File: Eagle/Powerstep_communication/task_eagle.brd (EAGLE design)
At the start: 82.5 x 123.6 mm, 104 parts, among them IC2 ATMEGA640-16AI, IC3 74ACT125D, IC7 FT232RL, IC8 MAX485, K1 G5LE, K2 G5LE, K3 G5LE, K6 G5LE, U1 TC1262-33VDB, U2 Tyco 5-6605758-1, U3 ENC28J60-SSOP, Y2 25MHz

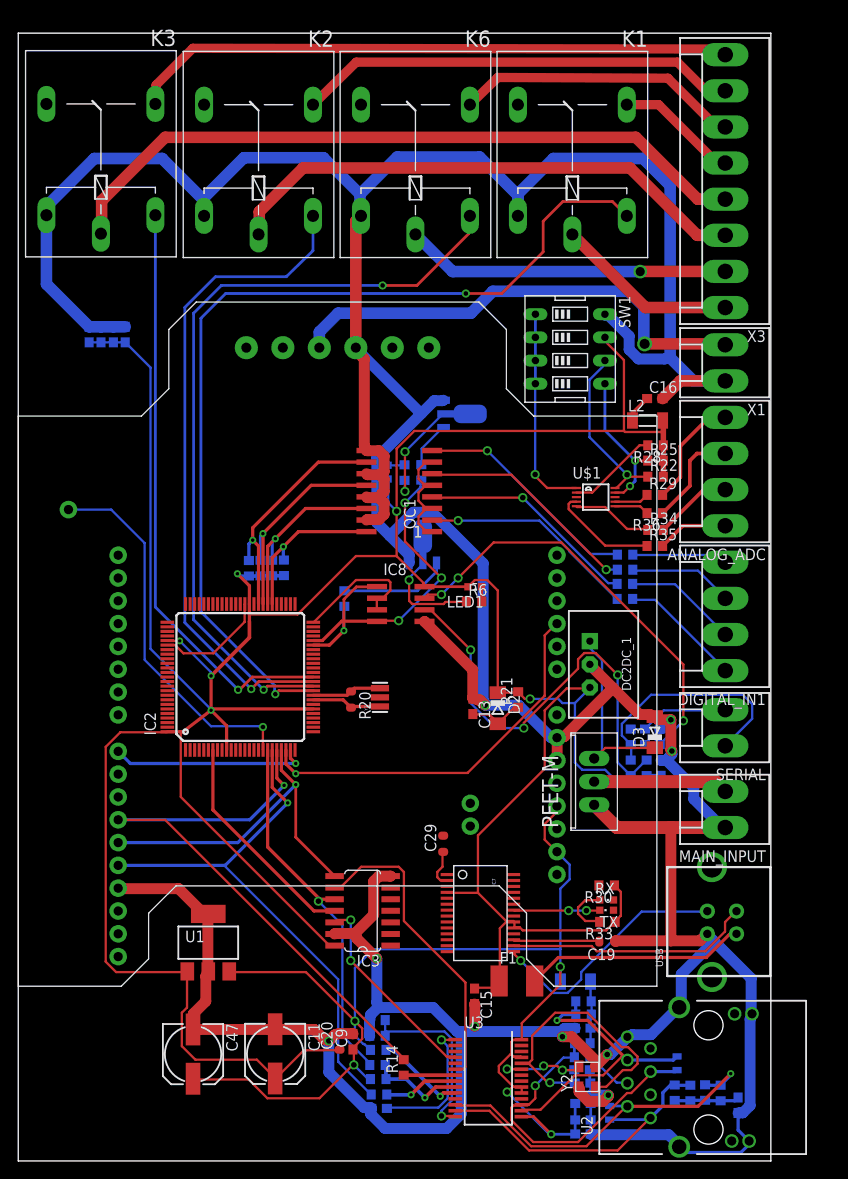
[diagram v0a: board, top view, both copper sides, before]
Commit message: eagle powerstepproto
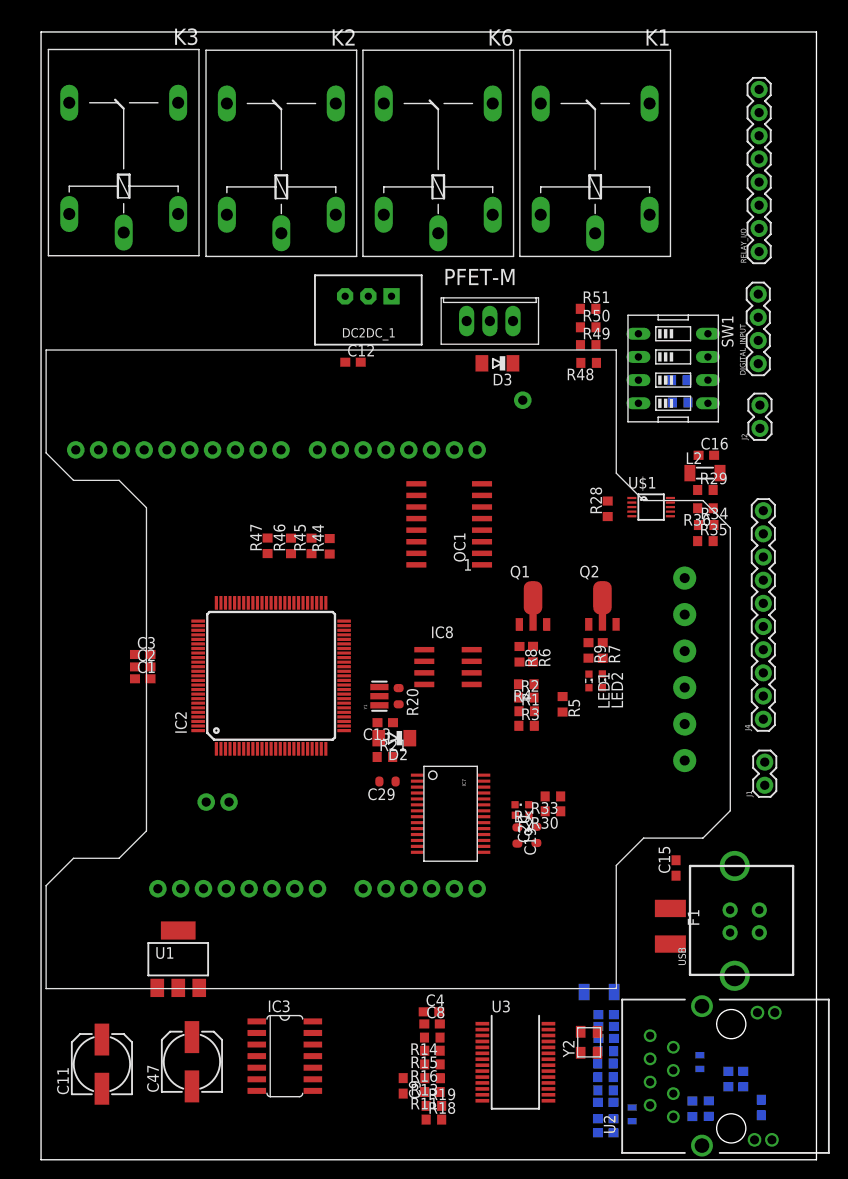
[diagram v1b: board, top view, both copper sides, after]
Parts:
- removed ANALOG_ADC, DIGITAL_IN1: (no value), con-molex:KK-156-4
- removed MAIN_INPUT, SERIAL, X1: (no value), con-molex:KK-156-2
- removed X3: (no value), con-molex:KK-156-8
- added DIGITAL_INPUT: (no value), SparkFun-Connectors:1X04
- added J1, J2: (no value), SparkFun-Connectors:1X02
- added J4: (no value), SparkFun-Connectors:1X10
- added RELAY_I/O: (no value), SparkFun-Connectors:1X08
- moved C4 81.5 mm to (42.8, 16.2), flipped to the top, turned to 0 degrees
- moved U$2 69.9 mm to (0.49, 88.8), turned to 270 degrees
- moved PFET-M 59.8 mm to (44.1, 94.5), turned to 0 degrees
- moved C12 55.9 mm to (34.2, 87.4), flipped to the top, turned to 0 degrees
- moved DC2DC_1 46.6 mm to (35.9, 93.2), turned to 180 degrees
- moved D3 44.0 mm to (50.0, 87.3), turned to 180 degrees
- moved C1 38.2 mm to (11.1, 52.7), flipped to the top, turned to 0 degrees
- moved C2 36.7 mm to (11.1, 54.0), flipped to the top, turned to 0 degrees
- moved C3 35.2 mm to (11.1, 55.4), flipped to the top, turned to 0 degrees
- moved LED2 32.8 mm to (61.5, 52.5), flipped to the top
- moved C20 31.3 mm to (54.3, 35.6)
- moved R7 29.2 mm to (61.6, 55.8), flipped to the top, turned to 270 degrees
- moved R51 27.3 mm to (60.0, 93.3), flipped to the top
- moved R50 26.9 mm to (60.0, 91.3), flipped to the top
- moved R9 26.8 mm to (60.0, 55.8), flipped to the top
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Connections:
- new net N$19: J4.1, U$2.A+
- new net N$33: J4.2, U$2.B+
- new net N$34: J4.5, U$2.B-
- new net N$35: J4.6, U$2.A-
- net 12V_IN: now also J2.2; no longer MAIN_INPUT.2
- net A: now also J1.1; no longer SERIAL.1
- net A0_ADC: now also J4.7; no longer ANALOG_ADC.1
- net A1_ADC: now also J4.8; no longer ANALOG_ADC.2
- net A2_ADC: now also J4.9; no longer ANALOG_ADC.3
- net A3_ADC: now also J4.10; no longer ANALOG_ADC.4
- net B: now also J1.2; no longer SERIAL.2
- net COMM_1: now also RELAY_I/O.1; no longer X3.1
- net COMM_2: now also RELAY_I/O.2; no longer X3.2
- net COMM_3: now also RELAY_I/O.3; no longer X3.3
- net COMM_4: now also RELAY_I/O.4; no longer X3.4
- net DIG1_48V: now also RELAY_I/O.5; no longer X3.5
- net DIG2_48V: now also RELAY_I/O.6; no longer X3.6
- net DIG3_48V: now also RELAY_I/O.7; no longer X3.7
- net DIG4_48V: now also RELAY_I/O.8; no longer X3.8
- net DIG_24V_IN_1: now also DIGITAL_INPUT.1; no longer DIGITAL_IN1.1
- net DIG_24V_IN_2: now also DIGITAL_INPUT.2; no longer DIGITAL_IN1.2
- net DIG_24V_IN_3: now also DIGITAL_INPUT.3; no longer DIGITAL_IN1.3
- net DIG_24V_IN_4: now also DIGITAL_INPUT.4; no longer DIGITAL_IN1.4
- net GND: now also J2.1, J4.3; no longer MAIN_INPUT.1, X1.1
- net RESET_1: now also IC2.63; no longer IC2.24
- net RESET_FTDI: now also IC2.5; no longer IC2.60
- net RX_FTDI: now also IC2.2; no longer IC2.63
- net TX_FTDI: now also IC2.3; no longer IC2.64
- net VMOT: now also J4.4; no longer X1.2
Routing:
- net GND: track 578.3 -> 0.00 mm, vias 9 -> 0
- net VCC: track 399.0 -> 0.00 mm, vias 6 -> 0
- net 3.3V: track 136.5 -> 0.00 mm, vias 5 -> 0
- net RELAY_1_IN: track 103.5 -> 0.00 mm, vias 2 -> 0
- net RELAY_2_IN: track 85.8 -> 0.00 mm, vias 2 -> 0
- net COMM_4: track 77.7 -> 0.00 mm
- net RELAY_3_IN: track 72.4 -> 0.00 mm, vias 1 -> 0
- net DIG4_48V: track 66.3 -> 0.00 mm
- net MOSI_1: track 66.3 -> 0.00 mm, vias 1 -> 0
- net RELAY_4_IN: track 64.7 -> 0.00 mm, vias 1 -> 0
- net SCK_1: track 59.7 -> 0.00 mm, vias 1 -> 0
- net COMM_3: track 58.6 -> 0.00 mm
- net VMOT: track 52.8 -> 0.00 mm, vias 1 -> 0
- net N$1: track 49.4 -> 0.00 mm, vias 3 -> 0
- net DIG3_48V: track 48.4 -> 0.00 mm
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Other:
- board size 82.5 x 123.6 mm -> 85 x 123.6 mm

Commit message: powerstep.brd
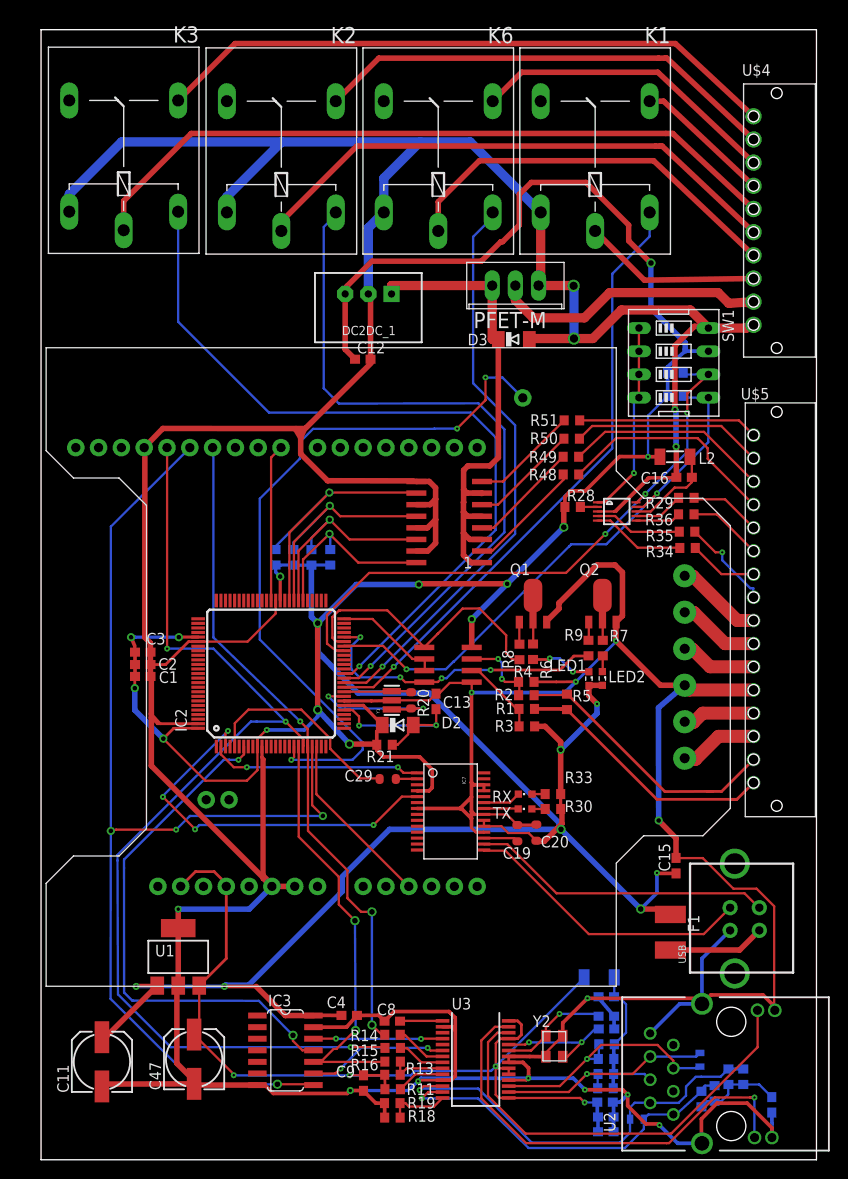
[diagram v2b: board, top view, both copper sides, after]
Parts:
- removed DIGITAL_INPUT: (no value), SparkFun-Connectors:1X04
- removed J1, J2: (no value), SparkFun-Connectors:1X02
- removed J4: (no value), SparkFun-Connectors:1X10
- removed RELAY_I/O: (no value), SparkFun-Connectors:1X08
- added U$4: 10_R44 - 1821326, Pheonix_connectors:10_R44 - 1821326
- added U$5: 16_R56 - 1821384, Pheonix_connectors:16_R56 - 1821384
- C1, C2, C3: value 100uF -> 100u
- moved PFET-M 13.0 mm to (57.1, 93.3), turned to 180 degrees
- moved R48 12.4 mm to (58.1, 75.1)
- moved R49 12.4 mm to (58.1, 77.1), turned to 180 degrees
- moved R51 12.4 mm to (58.2, 81.1), turned to 180 degrees
- moved R50 12.4 mm to (58.2, 79.0), turned to 180 degrees
- moved C4 9.03 mm to (33.8, 15.8)
- moved C13 6.03 mm to (43.3, 50.2), turned to 270 degrees
- moved R19 4.57 mm to (38.5, 6.21)
- moved R18 4.55 mm to (38.5, 4.62)
- moved R13 4.42 mm to (38.5, 9.32)
- moved C8 4.37 mm to (38.5, 15.2)
- moved C9 4.37 mm to (35.3, 8.41)
- moved R11 4.37 mm to (38.5, 7.74)
- moved R14 4.37 mm to (38.5, 13.7)
- moved R15 4.37 mm to (38.5, 12.3)
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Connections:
- removed net 12V_INPUT: OC1.1, OC1.3, OC1.5, OC1.7
- removed net N$19: J4.1, U$2.A+
- removed net N$33: J4.2, U$2.B+
- removed net N$34: J4.5, U$2.B-
- removed net N$35: J4.6, U$2.A-
- new net A+_STEP: U$2.A+, U$5.P$3
- new net A-_STEP: U$2.A-, U$5.P$8
- new net B+_STEP: U$2.B+, U$5.P$4
- new net B-_STEP: U$2.B-, U$5.P$7
- net 12V: now also OC1.1, OC1.3, OC1.5, OC1.7
- net 12V_IN: now also U$4.P$10; no longer J2.2
- net A: now also U$5.P$1; no longer J1.1
- net A0_ADC: now also U$5.P$9; no longer J4.7
- net A1_ADC: now also U$5.P$10; no longer J4.8
- net A2_ADC: now also U$5.P$11; no longer J4.9
- net A3_ADC: now also U$5.P$12; no longer J4.10
- net B: now also U$5.P$2; no longer J1.2
- net COMM_1: now also U$4.P$9; no longer RELAY_I/O.1
- net COMM_2: now also U$4.P$8; no longer RELAY_I/O.2
- net COMM_3: now also U$4.P$7; no longer RELAY_I/O.3
- net COMM_4: now also U$4.P$6; no longer RELAY_I/O.4
- net DIG1_48V: now also U$4.P$5; no longer RELAY_I/O.5
- net DIG2_48V: now also U$4.P$4; no longer RELAY_I/O.6
- net DIG3_48V: now also U$4.P$3; no longer RELAY_I/O.7
- net DIG4_48V: now also U$4.P$2; no longer RELAY_I/O.8
- net DIG_24V_IN_1: now also U$5.P$13; no longer DIGITAL_INPUT.1
- net DIG_24V_IN_2: now also U$5.P$14; no longer DIGITAL_INPUT.2
- net DIG_24V_IN_3: now also U$5.P$15; no longer DIGITAL_INPUT.3
- net DIG_24V_IN_4: now also U$5.P$16; no longer DIGITAL_INPUT.4
- net GND: now also U$4.P$11, U$5.P$5; no longer J2.1, J4.3
- net VMOT: now also U$5.P$6; no longer J4.4
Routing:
- net GND: track 0.00 -> 734.5 mm, vias 0 -> 16
- net VCC: track 0.00 -> 413.6 mm, vias 0 -> 22
- net MISO_1: track 0.00 -> 122.2 mm, vias 0 -> 4
- net SCK_1: track 0.00 -> 113.4 mm, vias 0 -> 3
- net 3.3V: track 0.00 -> 107.7 mm, vias 0 -> 4
- net RELAY_4_IN: track 0.00 -> 85.4 mm, vias 0 -> 1
- net CCW: track 0.00 -> 79.8 mm, vias 0 -> 3
- net COMM_4: track 0.00 -> 78.6 mm
- net RELAY_3_IN: track 0.00 -> 77.0 mm, vias 0 -> 1
- net MOSI_1: track 0.00 -> 73.2 mm, vias 0 -> 3
- net DIG4_48V: track 0.00 -> 69.4 mm
- net RELAY_1_IN: track 0.00 -> 67.8 mm, vias 0 -> 1
- net SCL_ADC: track 0.00 -> 66.0 mm, vias 0 -> 3
- net RELAY_2_IN: track 0.00 -> 63.5 mm, vias 0 -> 1
- net SDA_ADC: track 0.00 -> 62.1 mm, vias 0 -> 2
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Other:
- board size 85 x 123.6 mm -> 85 x 123.9 mm
